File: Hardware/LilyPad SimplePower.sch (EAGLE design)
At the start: 21 parts, among them U1 MCP73831

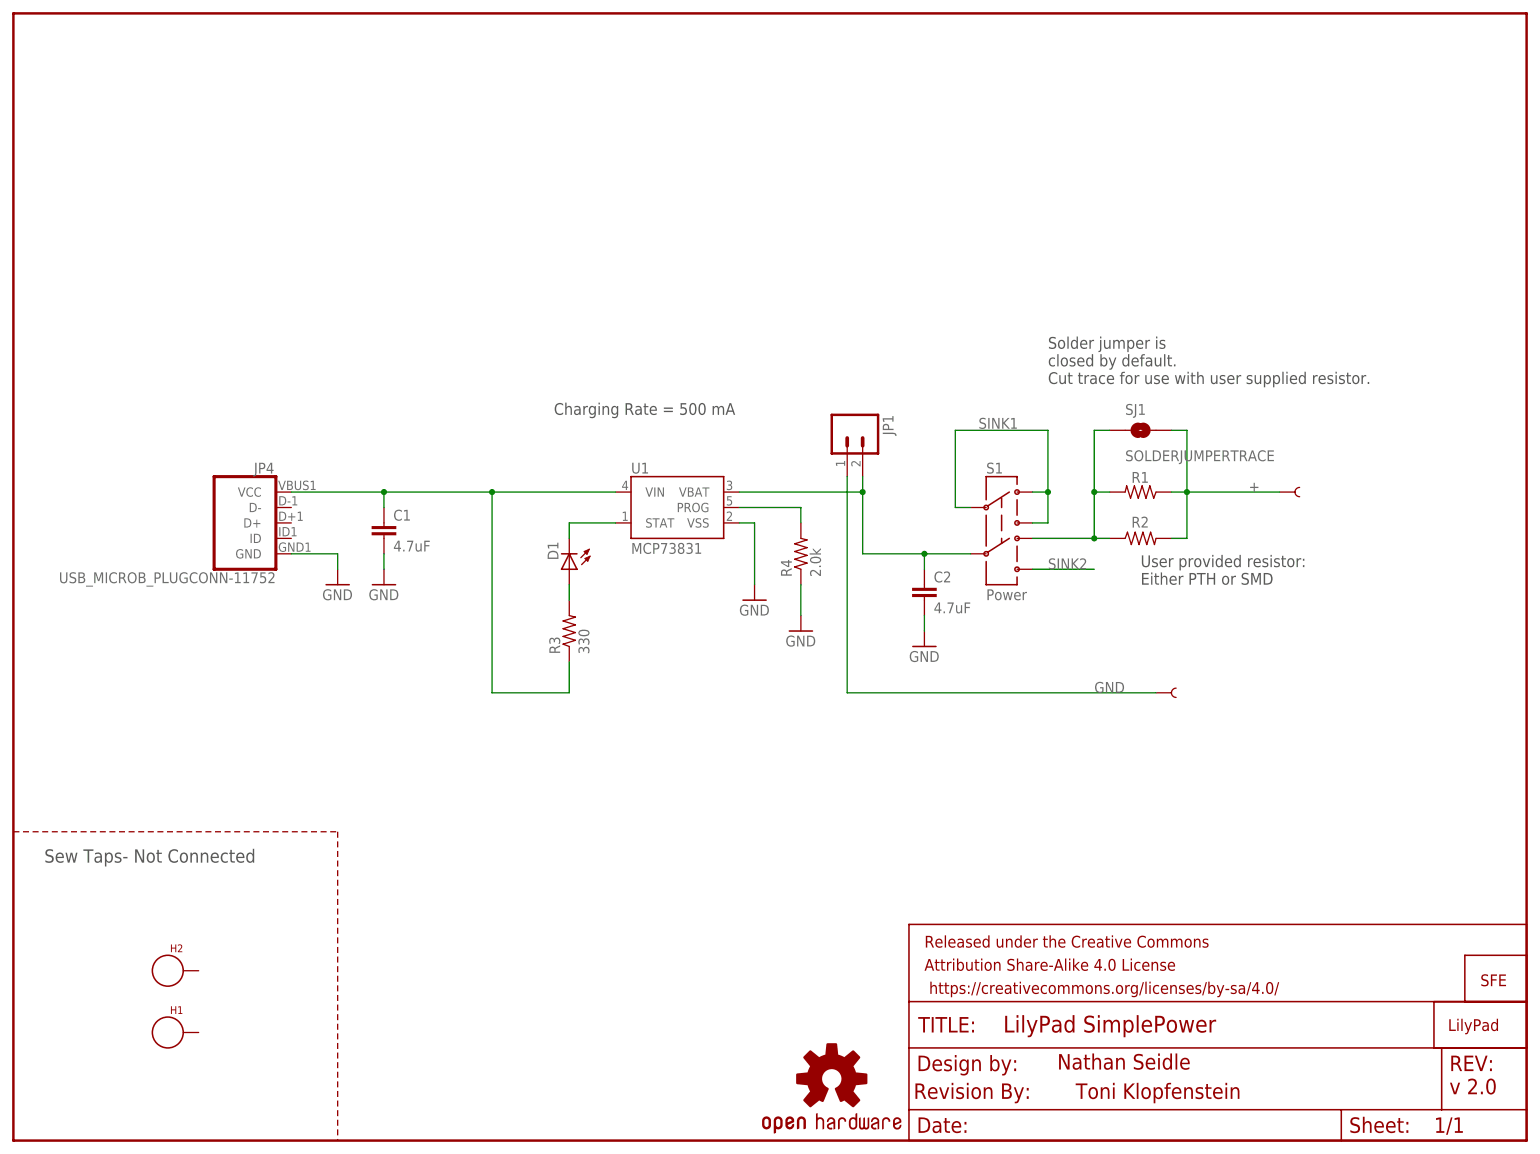
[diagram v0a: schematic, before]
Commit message: midway work  on updating design
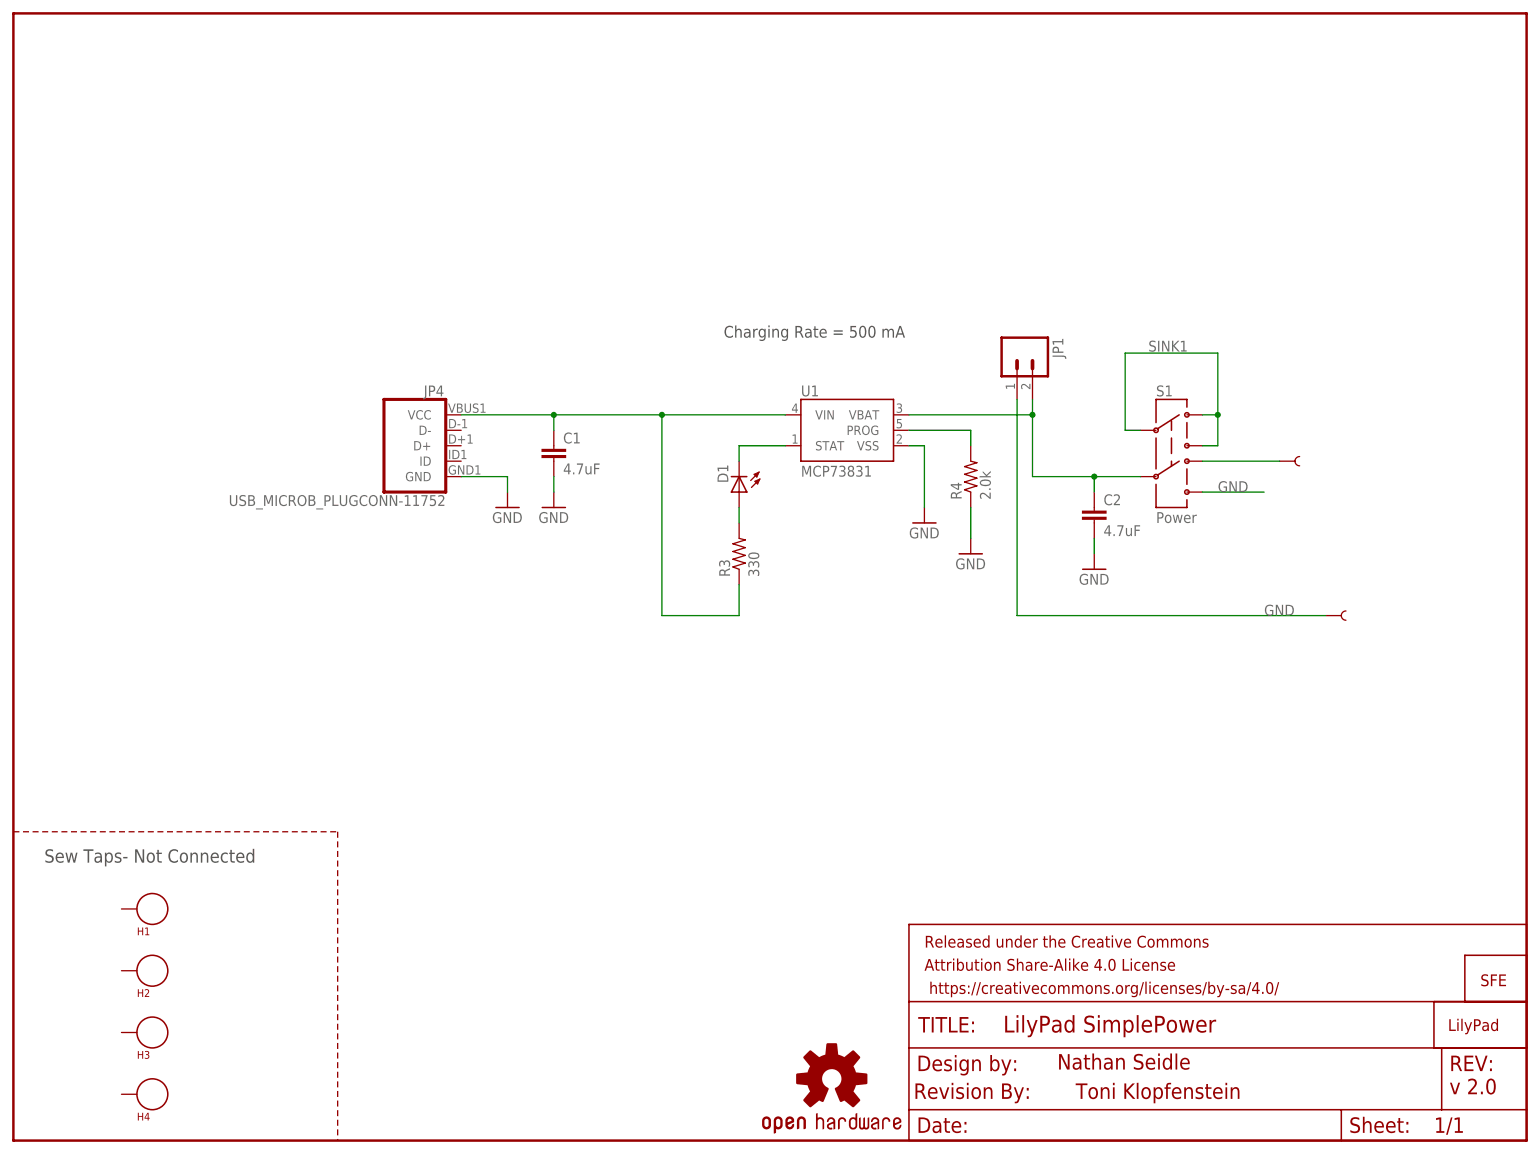
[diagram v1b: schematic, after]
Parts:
- removed R1: (no value), SparkFun:RESISTORAXIAL-0.3
- removed R2: (no value), SparkFun:RESISTOR1206
- removed SJ1: SOLDERJUMPERTRACE, SparkFun-Passives:SOLDERJUMPERTRACE
- added H3, H4: SEW_HOLE, LilyPad-Wearables:SEW_HOLE
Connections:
- removed net +: R1.1, R2.2, SJ1.2, U$4.1
- removed net N$2: R1.2, R2.1, S1.4, SJ1.1
- removed net SINK2: S1.6
- new net N$6: S1.4, U$4.1
- net GND: now also S1.6
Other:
- note removed: "Solder jumper is closed by default. Cut trace for use with user supplied resistor."
- note removed: "User provided resistor: Either PTH or SMD"
- moved on the sheet: C1, C2, D1, H1, H2, JP1, JP4, R3, R4, S1, U1
